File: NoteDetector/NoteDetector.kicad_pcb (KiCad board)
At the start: 2 copper layers, 25.4 x 25.4 mm, 49 parts, among them J1 Conn_01x01, J2 Conn_01x01, J3 Conn_01x01, J4 Conn_01x01, J5 Conn_01x01, J6 Conn_01x01, J7 Conn_01x01, Q1 Q_NMOS_DGS, Q2 Q_NMOS_DGS, Q3 Q_NMOS_DGS, Q4 Q_NMOS_DGS, U1 OPAMP, U2 PIC18F06

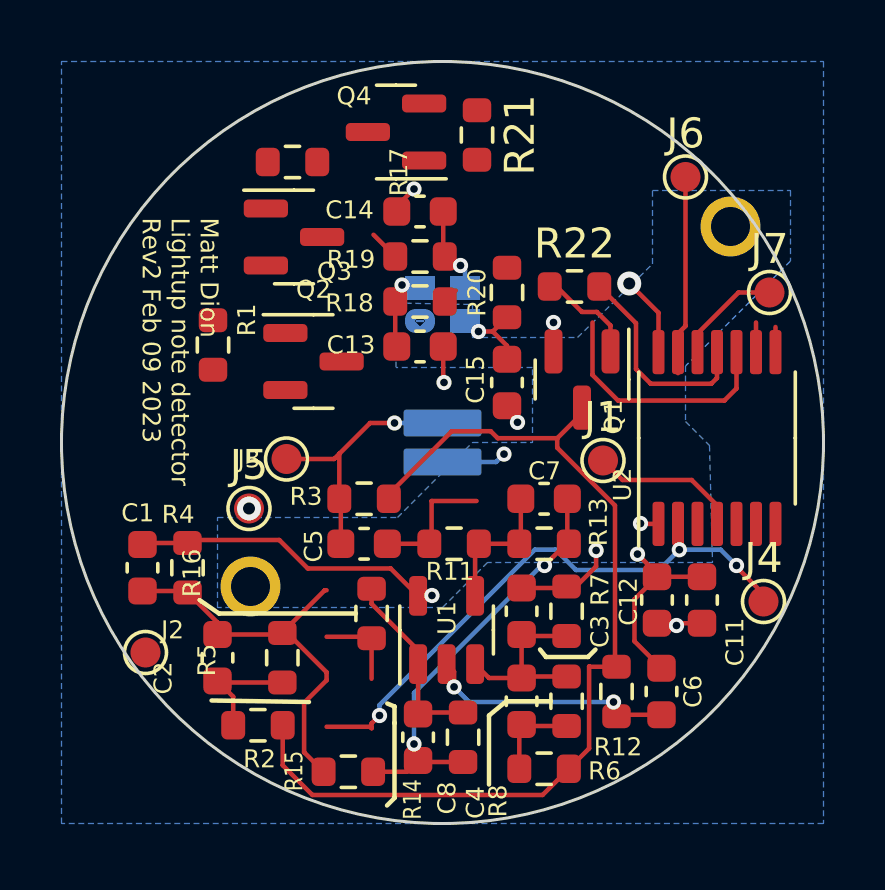
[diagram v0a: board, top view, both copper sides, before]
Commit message: Rev 3 layout (hastily) completed!
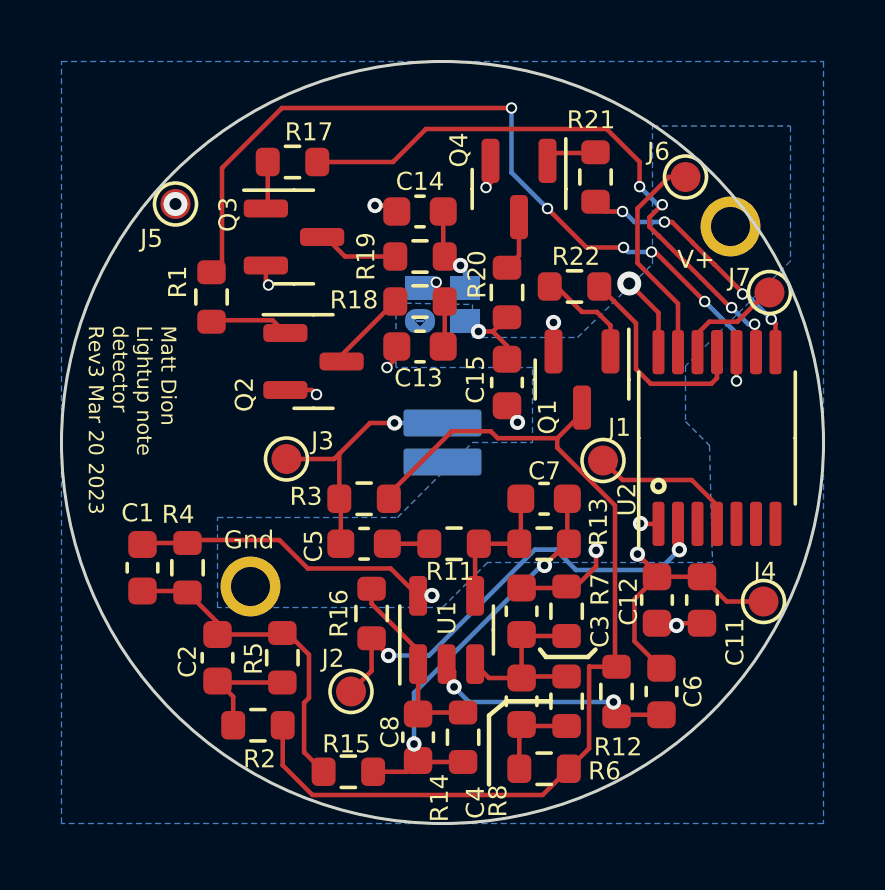
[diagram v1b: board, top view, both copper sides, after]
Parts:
- moved J5 10.4 mm to (-8.90, -7.95)
- moved J2 6.97 mm to (-3.05, 8.30)
- moved Q4 4.52 mm to (2.55, -8.45), turned to -90 degrees
- moved R21 4.19 mm to (5.10, -8.85), turned to 90 degrees
- moved R1 1.60 mm to (-7.70, -4.85), turned to 90 degrees
- turned C13 to 180 degrees
- turned R18 to 180 degrees
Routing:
- net /PWM1: track 8.28 -> 28.5 mm, vias 0 -> 6
- net /PWM2: track 0.99 -> 20.3 mm, vias 0 -> 4
- net /PWM3: track 1.46 -> 8.67 mm, vias 0 -> 4
- net /Audio_In: track 22.0 -> 15.5 mm, vias 3 -> 2
- net Net-(C5-Pad2): track 4.36 -> 1.51 mm
- net Net-(Q2-Pad1): track 0.00 -> 2.59 mm
- net /Midscale2: track 13.5 -> 10.9 mm
- net Net-(Q2-Pad3): track 0.51 -> 2.74 mm
- net Net-(Q4-Pad3): track 0.00 -> 1.85 mm
- net Net-(Q4-Pad1): track 0.00 -> 1.72 mm
- net Net-(Q3-Pad3): track 1.03 -> 2.71 mm
- net Net-(Q3-Pad1): track 0.00 -> 1.58 mm
- net GND: track 8.73 -> 10.3 mm, vias 7 -> 10
- net /ICSP_DAT: track 6.64 -> 8.00 mm
- net /ICSP_CLK: track 4.20 -> 3.59 mm
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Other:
- board text added: "Gnd"
- board text added: "Matt Dion Lightup note detector Rev3 Mar 20 2023"
- board text added: "V+"
- board text removed: "Matt Dion Lightup note detector Rev2 Feb 09 2023"
